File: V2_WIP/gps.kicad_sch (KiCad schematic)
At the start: 23 parts, among them U102 *W25Q128JFV, U103 ICM-45686

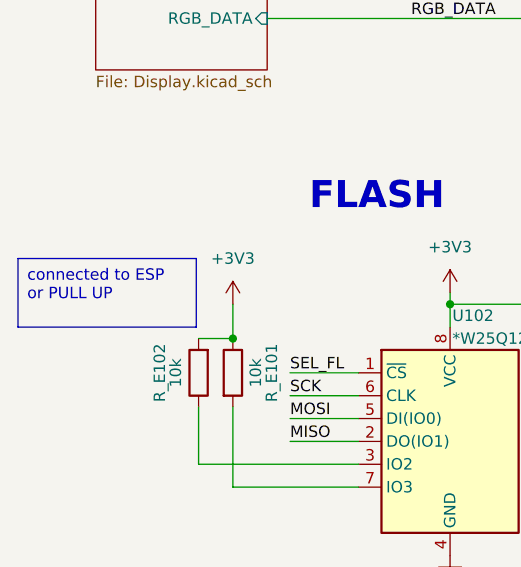
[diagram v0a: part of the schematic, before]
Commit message: up to date i dont remember what changed
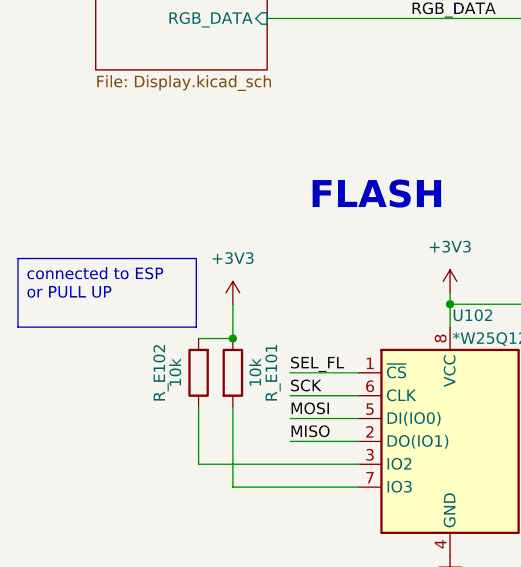
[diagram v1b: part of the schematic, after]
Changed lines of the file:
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@@
 (kicad_sch
-	(version 20231120)
+	(version 20250114)
 	(generator "eeschema")
-	(generator_version "8.0")
+	(generator_version "9.0")
 	(paper "A4")
 	(title_block
@@
 		(rev "1")
 	)
+	(text "ESP module"
+		(exclude_from_sim no)
+		(at 208.28 17.78 0)
+		(effects
+			(font
+				(size 3 3)
+				(bold yes)
+			)
+		)
+	)
+	(text "FLASH"
+		(exclude_from_sim no)
+		(at 60.452 140.462 0)
+		(effects
+			(font
+				(size 3 3)
+				(bold yes)
+			)
+		)
+	)
+	(text "IMU"
+		(exclude_from_sim no)
+		(at 132.334 138.938 0)
+		(effects
+			(font
+				(size 3 3)
+				(bold yes)
+			)
+		)
+	)
+	(text_box "connected to ESP or PULL UP"
+		(exclude_from_sim no)
+		(at 20.574 147.32 0)
+		(size 19.812 7.62)
+		(margins 0.9525 0.9525 0.9525 0.9525)
+		(stroke
+			(width 0)
+			(type default)
+		)
+		(fill
+			(type none)
+		)
+		(effects
+			(font
+				(size 1.27 1.27)
+			)
+			(justify left top)
+		)
+	)
 	(junction
 		(at 158.75 86.36)
@@
 		)
 	)
-	(text_box "connected to ESP or PULL UP"
-		(exclude_from_sim no)
-		(at 20.574 147.32 0)
-		(size 19.812 7.62)
-		(stroke
-			(width 0)
-			(type default)
-		)
-		(fill
-			(type none)
-		)
-		(effects
-			(font
-				(size 1.27 1.27)
-			)
-			(justify left top)
-		)
-	)
-	(text "ESP module"
-		(exclude_from_sim no)
-		(at 208.28 17.78 0)
-		(effects
-			(font
-				(size 3 3)
-				(bold yes)
-			)
-		)
-	)
-	(text "FLASH"
-		(exclude_from_sim no)
-		(at 60.452 140.462 0)
-		(effects
-			(font
-				(size 3 3)
-				(bold yes)
-			)
-		)
-	)
-	(text "IMU"
-		(exclude_from_sim no)
-		(at 132.334 138.938 0)
-		(effects
-			(font
-				(size 3 3)
-				(bold yes)
-			)
-		)
-	)
 	(label "SW"
 		(at 181.61 54.61 0)
-		(fields_autoplaced yes)
 		(effects
 			(font
@@
 	(label "DT"
 		(at 181.61 62.23 0)
-		(fields_autoplaced yes)
 		(effects
 			(font
@@
 	(label "MISO"
 		(at 181.61 93.98 0)
-		(fields_autoplaced yes)
 		(effects
 			(font
@@
 	(label "MISO"
 		(at 111.76 160.02 0)
-		(fields_autoplaced yes)
 		(effects
 			(font
@@
 	(label "VBATT"
 		(at 181.61 67.31 0)
-		(fields_autoplaced yes)
 		(effects
 			(font
@@
 	(label "SCL_3V3"
 		(at 181.61 74.93 0)
-		(fields_autoplaced yes)
 		(effects
 			(font
@@
 	(label "MOSI"
 		(at 124.46 148.59 0)
-		(fields_autoplaced yes)
 		(effects
 			(font
@@
 	(label "SCK"
 		(at 50.8 162.56 0)
-		(fields_autoplaced yes)
 		(effects
 			(font
@@
 	(label "MOSI"
 		(at 50.8 165.1 0)
-		(fields_autoplaced yes)
 		(effects
 			(font
@@
 	(label "MISO"
 		(at 50.8 167.64 0)
-		(fields_autoplaced yes)
 		(effects
 			(font
@@
 	(label "CLK"
 		(at 181.61 58.42 0)
-		(fields_autoplaced yes)
 		(effects
 			(font
@@
 	(label "SEL_IMU"
 		(at 181.61 83.82 0)
-		(fields_autoplaced yes)
 		(effects
 			(font
@@
 	(label "SDA_3V3"
 		(at 181.61 77.47 0)
-		(fields_autoplaced yes)
 		(effects
 			(font
@@
 	(label "SEL_FL"
 		(at 50.8 160.02 0)
-		(fields_autoplaced yes)
 		(effects
 			(font
@@
 	(label "LIGHT_SENS"
 		(at 236.22 53.34 180)
-		(fields_autoplaced yes)
 		(effects
 			(font
@@
 	(label "SEL_IMU"
 		(at 124.46 143.51 0)
-		(fields_autoplaced yes)
 		(effects
 			(font
@@
 	(label "GNSS_TxD"
 		(at 181.61 35.56 0)
-		(fields_autoplaced yes)
 		(effects
 			(font
@@
 	(label "SCK"
 		(at 181.61 88.9 0)
-		(fields_autoplaced yes)
 		(effects
 			(font
@@
 	(label "SCK"
 		(at 124.46 146.05 0)
-		(fields_autoplaced yes)
 		(effects
 			(font
@@
 	(label "MOSI"
 		(at 181.61 91.44 0)
-		(fields_autoplaced yes)
 		(effects
 			(font
@@
 	(label "Pulse"
 		(at 181.61 30.48 0)
-		(fields_autoplaced yes)
 		(effects
 			(font
@@
 	(label "VUSB"
 		(at 181.61 27.94 0)
-		(fields_autoplaced yes)
 		(effects
 			(font
@@
 	(label "VUSB"
 		(at 185.42 132.08 0)
-		(fields_autoplaced yes)
 		(effects
 			(font
@@
 	(label "GNSS_RxD"
 		(at 181.61 38.1 0)
-		(fields_autoplaced yes)
 		(effects
 			(font
@@
 	(label "RGB_DATA"
 		(at 73.66 120.65 180)
-		(fields_autoplaced yes)
 		(effects
 			(font
@@
 	(label "LIGHT_SENS"
 		(at 243.84 144.78 0)
-		(fields_autoplaced yes)
 		(effects
 			(font
@@
 	(label "SEL_FL"
 		(at 181.61 86.36 0)
-		(fields_autoplaced yes)
 		(effects
 			(font
@@
 		(at 29.845 73.66)
 		(size 22.225 19.05)
+		(exclude_from_sim no)
+		(in_bom yes)
+		(on_board yes)
+		(dnp no)
 		(fields_autoplaced yes)
 		(stroke
@@
 		(at 29.845 26.67)
 		(size 22.225 15.875)
+		(exclude_from_sim no)
+		(in_bom yes)
+		(on_board yes)
+		(dnp no)
 		(fields_autoplaced yes)
 		(stroke
@@
 		(at 29.21 51.435)
 		(size 22.86 13.97)
+		(exclude_from_sim no)
+		(in_bom yes)
+		(on_board yes)
+		(dnp no)
 		(fields_autoplaced yes)
 		(stroke
@@
 		(at 29.21 102.235)
 		(size 19.05 24.13)
+		(exclude_from_sim no)
+		(in_bom yes)
+		(on_board yes)
+		(dnp no)
 		(fields_autoplaced yes)
 		(stroke
@@
 		(at 196.85 24.892)
 		(size 25.4 72.898)
+		(exclude_from_sim no)
+		(in_bom yes)
+		(on_board yes)
+		(dnp no)
 		(fields_autoplaced yes)
 		(stroke
@@
 		(at 100.33 98.425)
 		(size 30.48 13.335)
+		(exclude_from_sim no)
+		(in_bom yes)
+		(on_board yes)
+		(dnp no)
 		(fields_autoplaced yes)
 		(stroke
@@
 		)
 	)
+	(embedded_fonts no)
 )
